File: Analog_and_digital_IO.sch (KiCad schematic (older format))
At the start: 106 parts

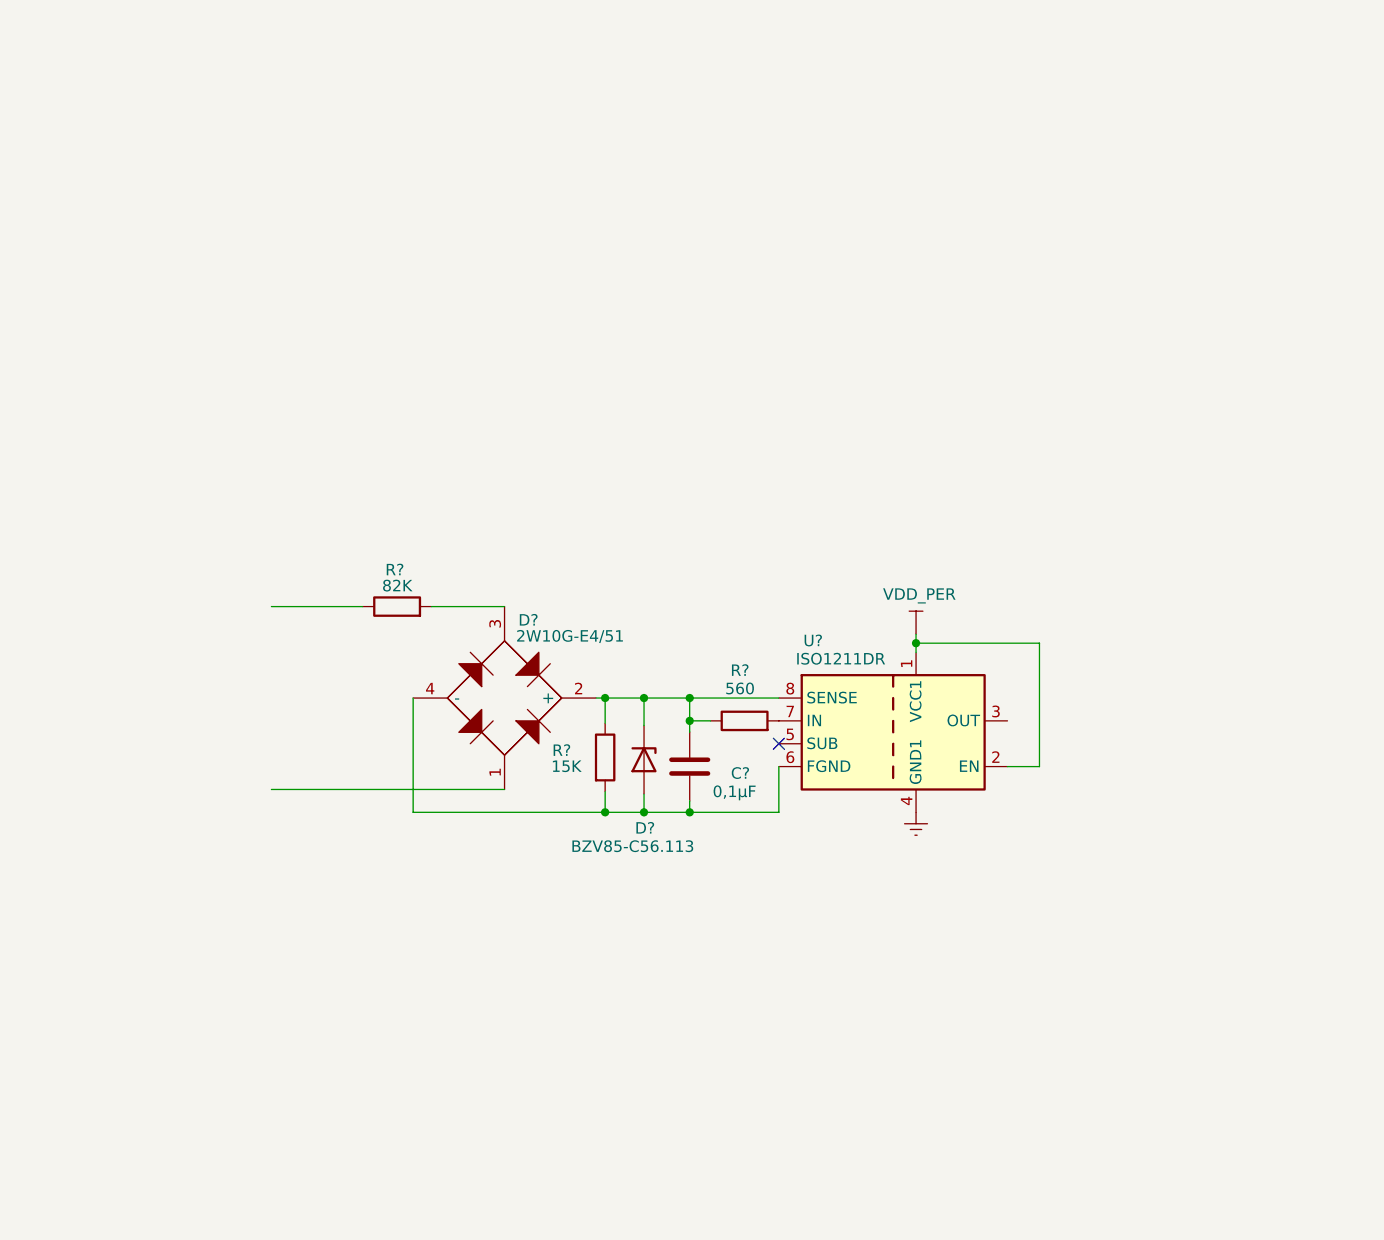
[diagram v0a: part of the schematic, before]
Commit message: Digital IO ended
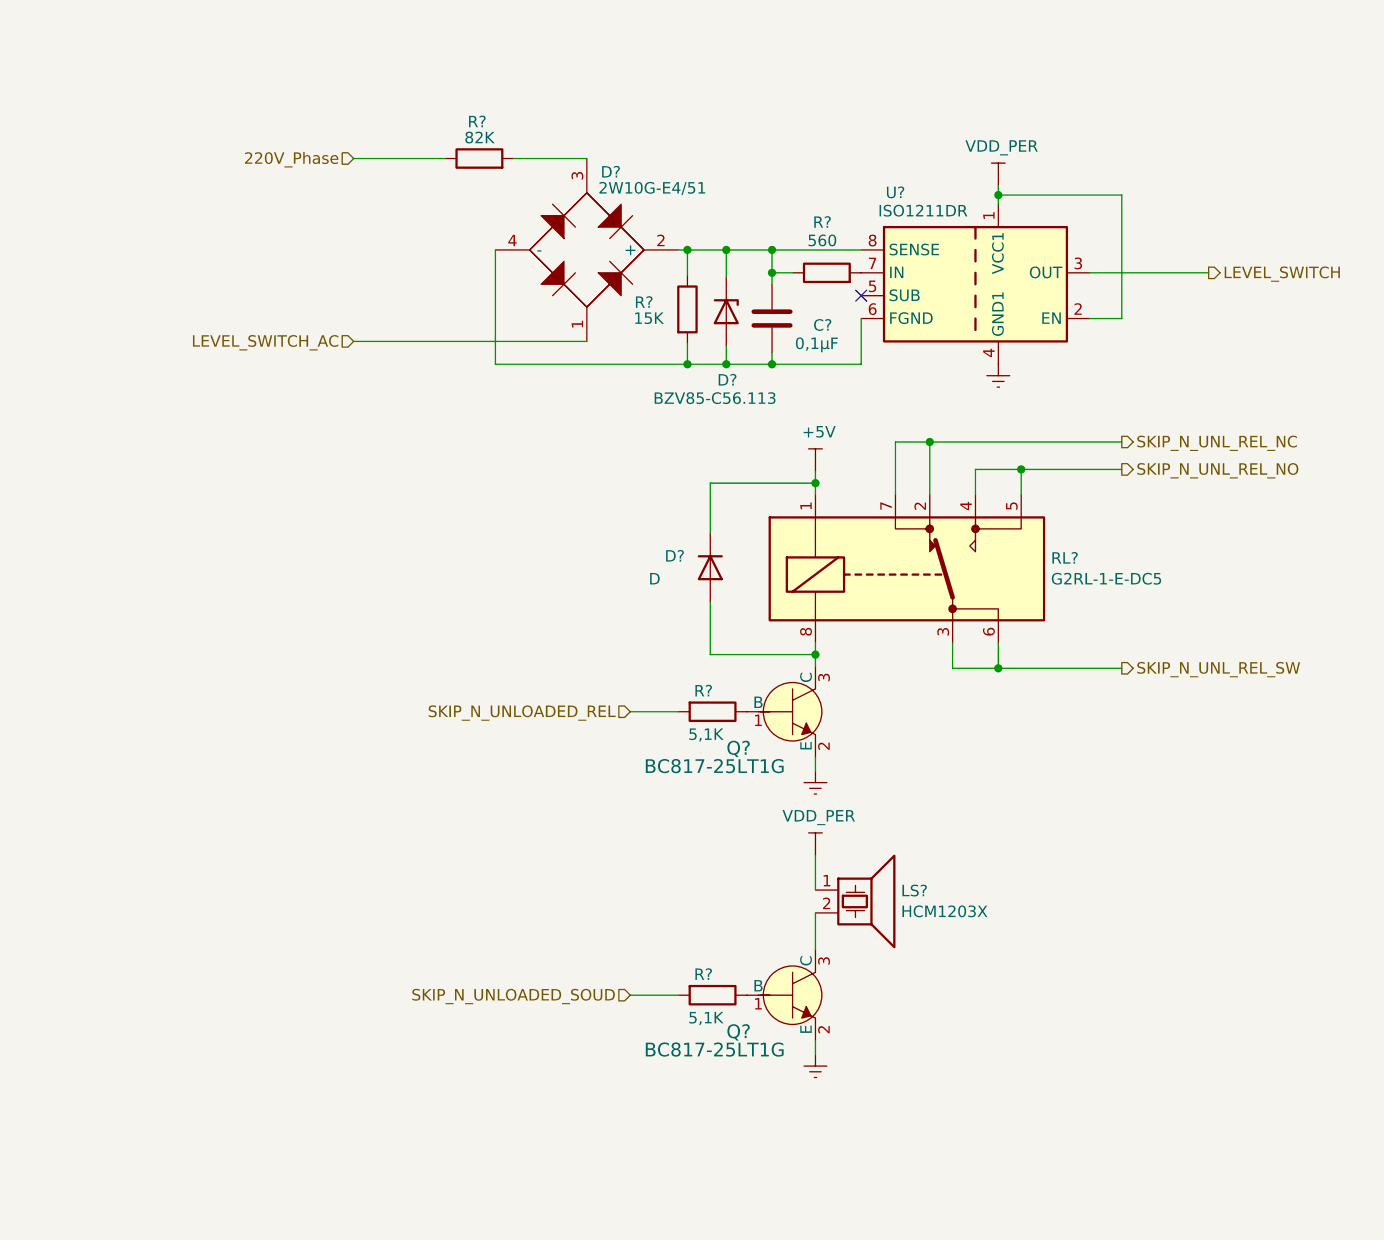
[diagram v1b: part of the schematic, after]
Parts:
- added D?: D, symbol Device:D
- added LS?: HCM1203X, symbol Device:Speaker_Crystal
- added Q? (x2): BC817-25LT1G, digikey-footprints:SOT-23-3, symbol dk_Transistors-Bipolar-BJT-Single:BC817-25LT1G
- added R? (x2): 5,1K, Resistor_SMD:R_0805_2012Metric_Pad1.20x1.40mm_HandSolder, symbol Device:R
- added RL?: G2RL-1-E-DC5, Relay_THT:Relay_DPDT_Omron_G2RL, symbol SVIELCOM_Library:G2RL-1-E-DC5
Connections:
- net GNDREF: now also Q?.2 (E), Q?.2 (E)
- net VDD_PER: now also LS?.1
- net 220V_Phase: now reaches R?.1
- net LEVEL_SWITCH: now reaches U?.3 (OUT)
- net LEVEL_SWITCH_AC: now reaches D?.1
- new net: Q?.1 (B), R?.1 (x2)
- new net: D?.2 (A), Q?.3 (C), RL?.8
- new net: LS?.2, Q?.3 (C)
- new net +5V: D?.1 (K), RL?.1
- new net SKIP_N_UNLOADED_REL: R?.2
- new net SKIP_N_UNLOADED_SOUD: R?.2
- new net SKIP_N_UNL_REL_NC: RL?.2, RL?.7
- new net SKIP_N_UNL_REL_NO: RL?.4, RL?.5
- new net SKIP_N_UNL_REL_SW: RL?.3, RL?.6
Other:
- moved on the sheet: C?, D?, R?, U?
